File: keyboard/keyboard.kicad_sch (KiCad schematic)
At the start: 138 parts, among them J1 Conn_01x04_Pin, J2 Conn_01x04_Pin, J3 Conn_01x04_Pin, J4 Conn_01x04_Pin, J5 Conn_01x04_Pin, J6 Conn_01x04_Pin, SW1 SW_Push, SW10 SW_Push, SW11 SW_Push, SW12 SW_Push, SW13 SW_Push, SW14 SW_Push, SW15 SW_Push, SW16 SW_Push, SW17 SW_Push, SW18 SW_Push, SW19 SW_Push, SW2 SW_Push, SW20 SW_Push, SW21 SW_Push, SW22 SW_Push, SW23 SW_Push, SW24 SW_Push, SW25 SW_Push, SW26 SW_Push, SW27 SW_Push, SW28 SW_Push, SW29 SW_Push, SW3 SW_Push, SW30 SW_Push, SW31 SW_Push, SW32 SW_Push, SW33 SW_Push, SW34 SW_Push, SW35 SW_Push, SW36 SW_Push, SW37 SW_Push, SW38 SW_Push, SW39 SW_Push, SW4 SW_Push, SW40 SW_Push, SW41 SW_Push, SW42 SW_Push, SW43 SW_Push, SW44 SW_Push, SW45 SW_Push, SW46 SW_Push, SW47 SW_Push, SW48 SW_Push, SW49 SW_Push, SW5 SW_Push, SW50 SW_Push, SW51 SW_Push, SW52 SW_Push, SW53 SW_Push, SW54 SW_Push, SW55 SW_Push, SW56 SW_Push, SW57 SW_Push, SW58 SW_Push, SW59 SW_Push, SW6 SW_Push, SW60 SW_Push, SW61 SW_Push, SW62 RotaryEncoder_Switch, SW7 SW_Push, SW8 SW_Push, SW9 SW_Push

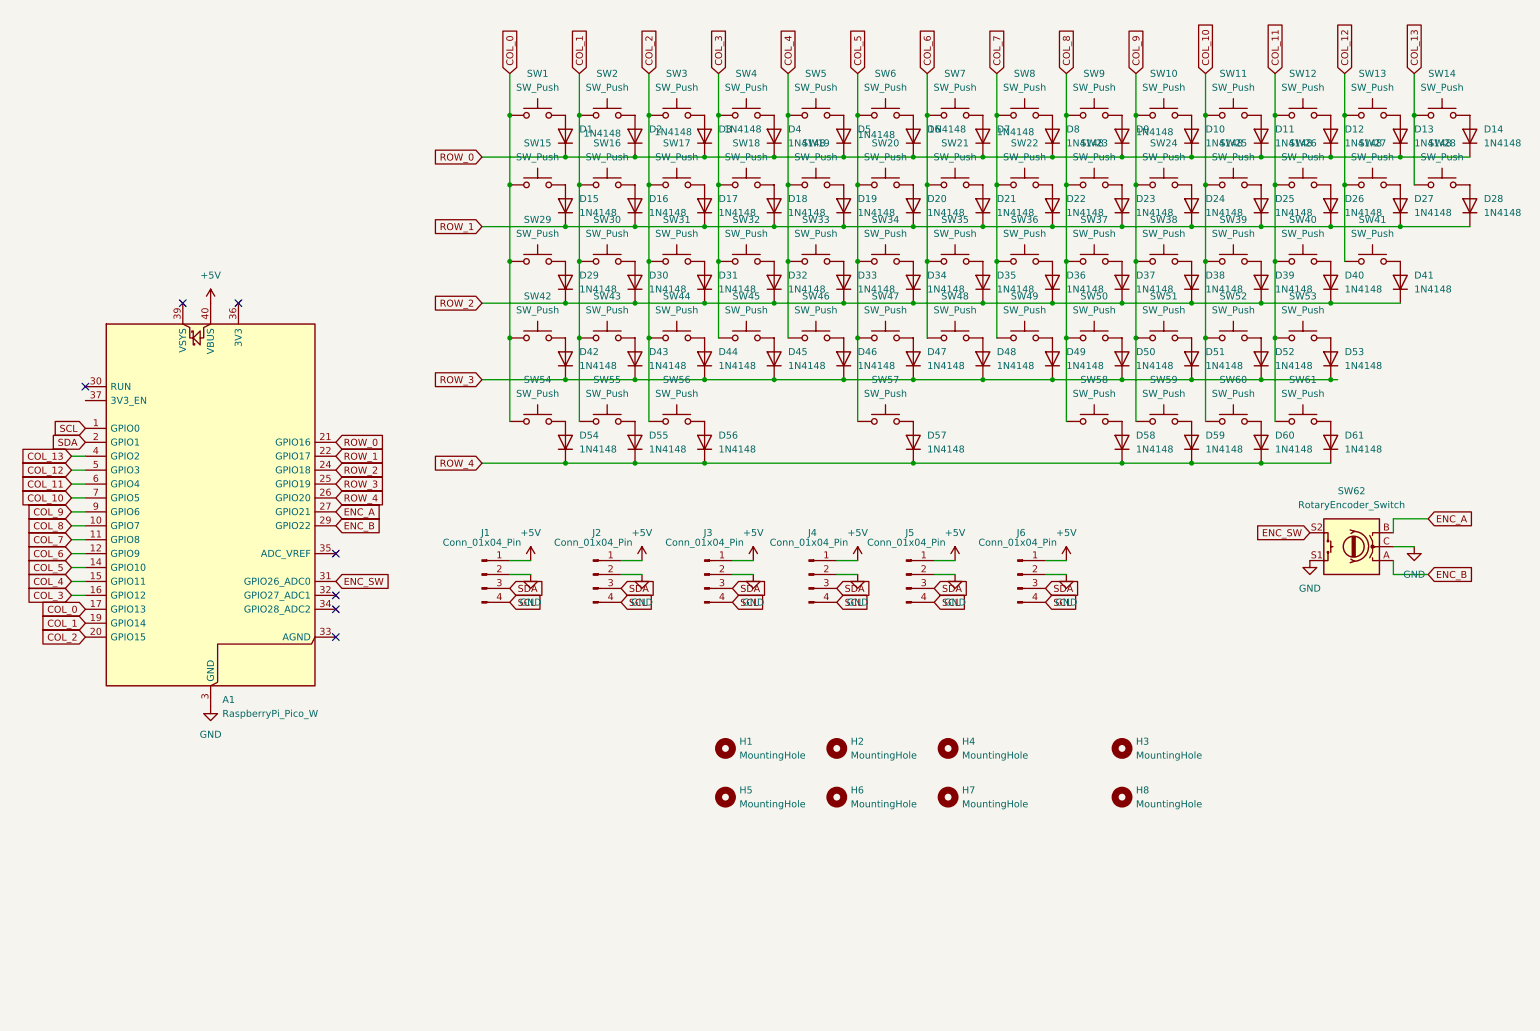
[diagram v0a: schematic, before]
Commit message: updates
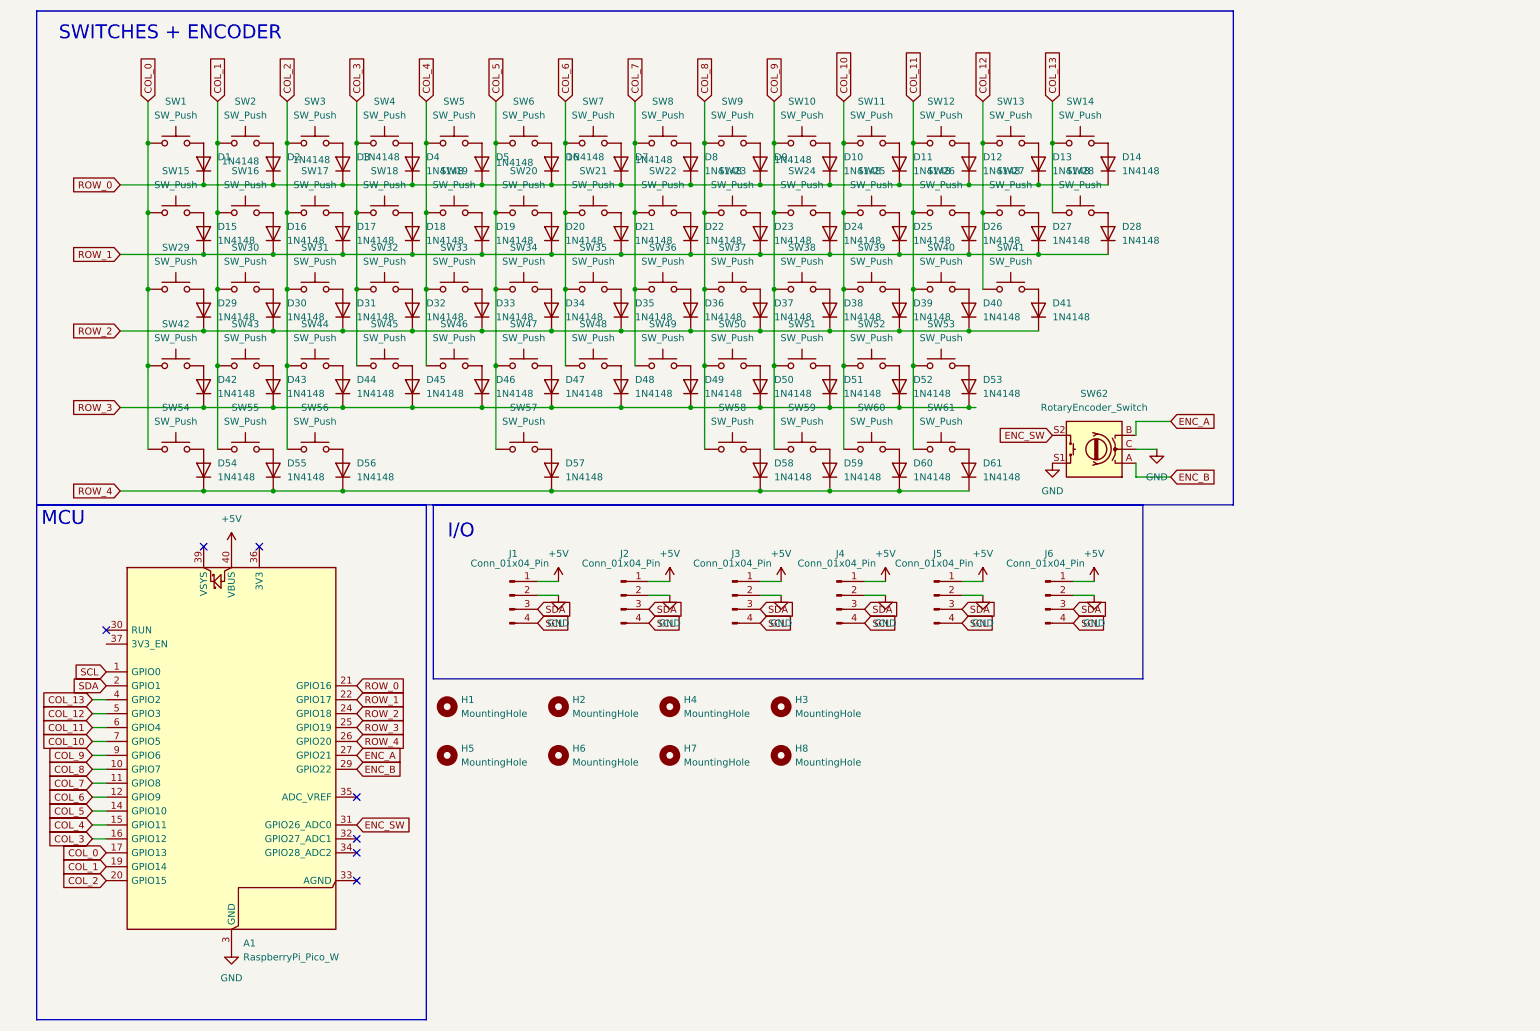
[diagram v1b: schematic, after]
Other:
- note added: "I/O"
- note added: "MCU"
- note added: "SWITCHES + ENCODER"
- moved on the sheet: A1, D1, D10, D11, D12, D13, D14, D15, D16, D17, D18, D19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
